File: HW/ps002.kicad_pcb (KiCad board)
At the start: 2 copper layers, 20 parts, among them J1 USB, J2 OUT, U1 MC34063

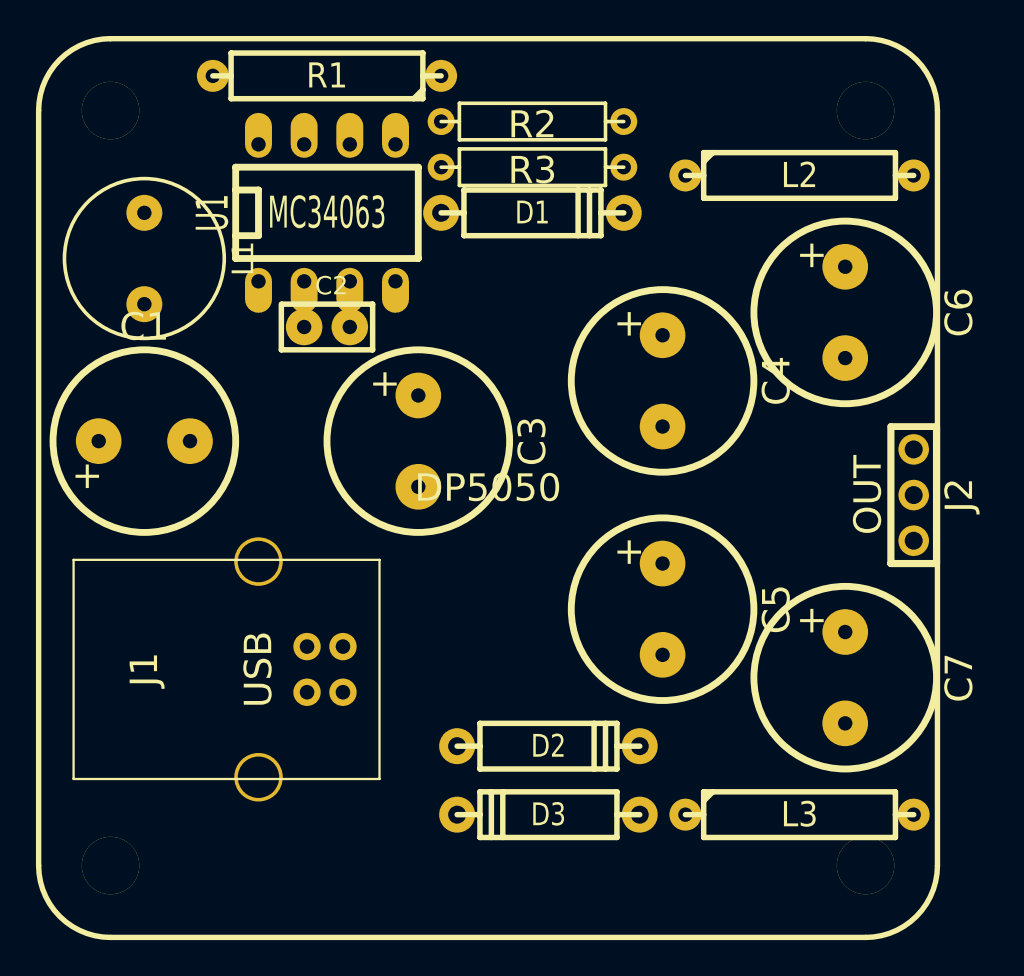
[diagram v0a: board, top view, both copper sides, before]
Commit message: PCB Routed
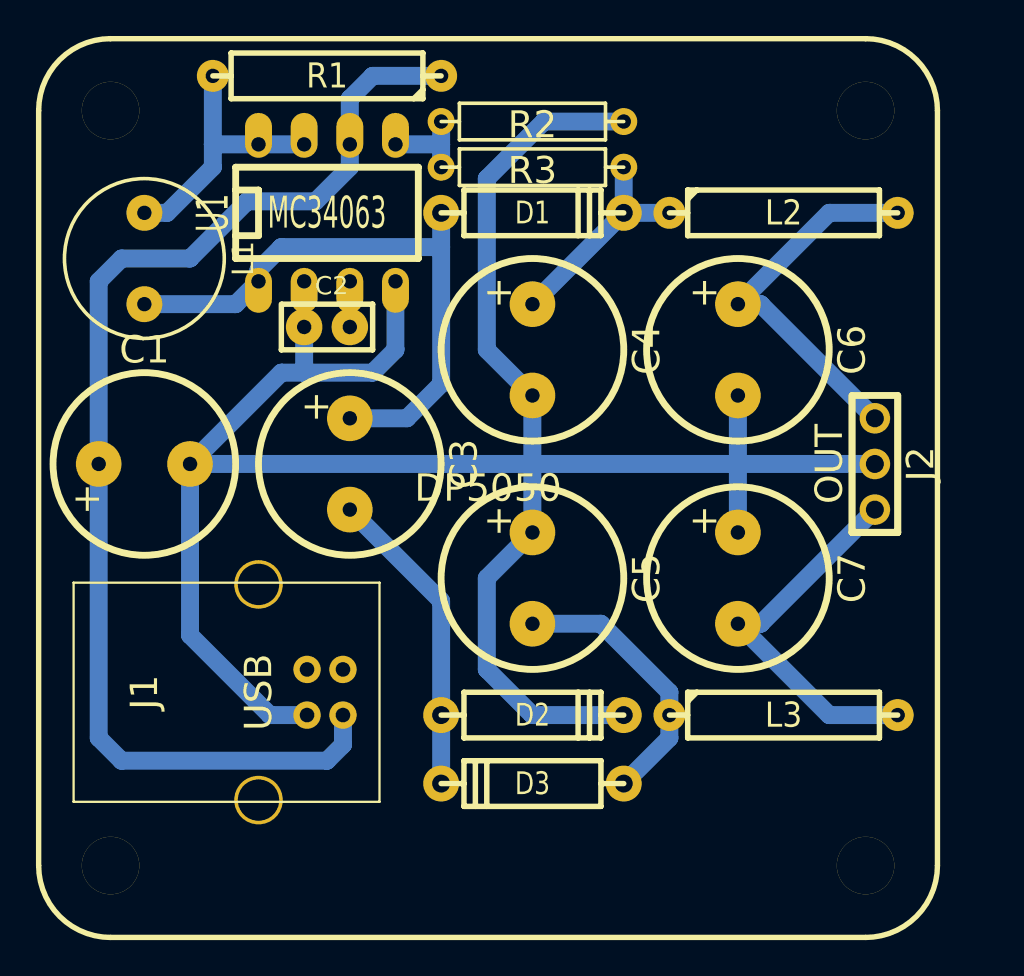
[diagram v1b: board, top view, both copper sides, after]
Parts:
- moved C7 8.14 mm to (88.9, 80.0)
- moved C4 7.44 mm to (77.5, 67.3)
- moved C5 7.44 mm to (77.5, 80.0)
- moved C6 6.32 mm to (88.9, 67.3)
- moved L3 5.61 mm to (91.4, 87.6)
- moved C3 4.02 mm to (67.3, 73.7)
- moved J2 2.77 mm to (96.5, 73.7)
- moved L2 2.26 mm to (91.4, 59.7)
- moved D2 1.95 mm to (77.5, 87.6)
- moved D3 1.95 mm to (77.5, 91.4)
- moved C1 1.27 mm to (55.9, 73.7)
- moved J1 1.27 mm to (62.2, 86.4)
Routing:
- net GND: track 2.54 -> 133.6 mm
- net VCC: track 0.00 -> 67.6 mm
- net N-000004: track 0.00 -> 33.6 mm
- net N-0000011: track 0.00 -> 21.2 mm
- net N-0000010: track 0.00 -> 21.2 mm
- net N-000003: track 0.00 -> 17.3 mm
- net N-0000012: track 0.00 -> 15.3 mm
- net N-0000015: track 0.00 -> 15.0 mm
- net N-0000013: track 0.00 -> 12.3 mm
- net N-000002: track 0.00 -> 5.08 mm
